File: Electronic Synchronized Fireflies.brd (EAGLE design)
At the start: 100 x 80 mm, 34 parts, among them Q1 NPN/PNP, U2 MSP430G2231/TSSOP-14, X1 22-23-2021, X2 22-23-2031

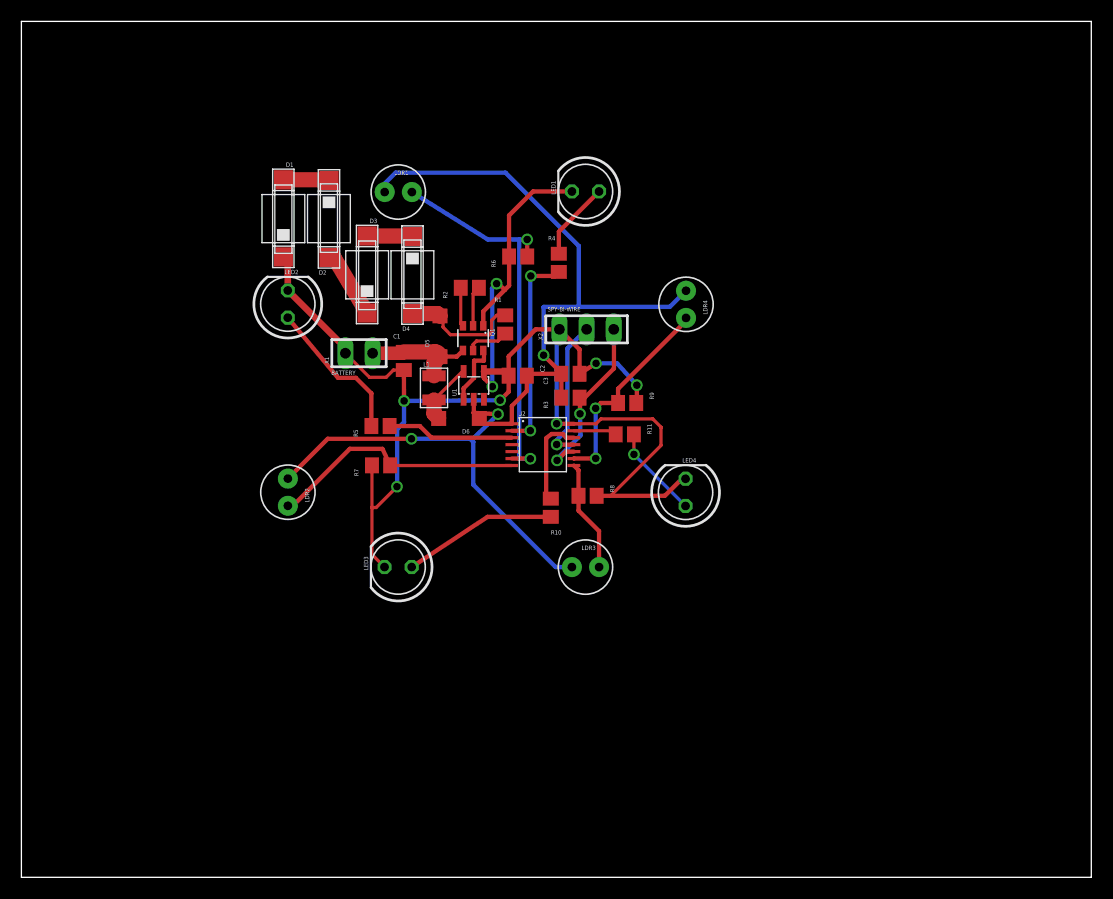
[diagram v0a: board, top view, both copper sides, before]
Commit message: Connections for panel, battery, PCB improvements
v0.3 EECS 399 Spring 2012
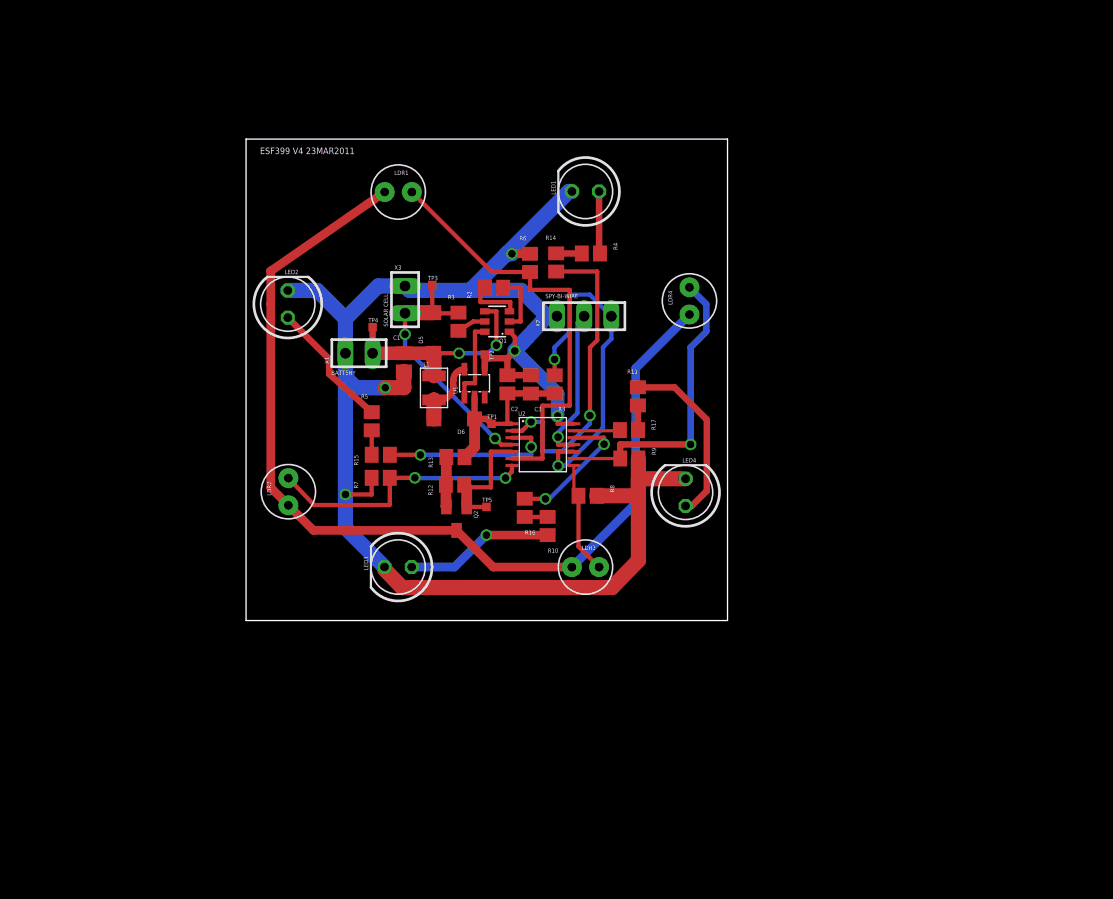
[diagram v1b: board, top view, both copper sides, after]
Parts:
- removed D1, D2, D3, D4: PHOTODIODESMD2, Firefly:PHOTODIODE-SMD2
- added Q2: DMP2035U-7, Firefly:SOT23
- added R12: 20kohm, Firefly:R0805
- added R13, R14, R15, R16, R17: 0ohm, Firefly:R0805
- added TP1, TP2, TP3, TP4, TP5: TPTP08SQ, Firefly:TP08SQ
- added X3: 22-23-2021, Firefly:22-23-2021
- moved R9 5.20 mm to (56.8, 39.1)
- moved R1 4.38 mm to (40.8, 51.9)
- moved C3 3.83 mm to (47.6, 46.1), turned to 90 degrees
- moved R11 3.76 mm to (57.6, 45.0), turned to 270 degrees
- moved R4 3.12 mm to (53.2, 58.3), turned to 180 degrees
- moved Q1 2.73 mm to (44.5, 52.0), turned to 90 degrees
- moved R2 2.27 mm to (44.2, 55.1)
- moved R3 1.93 mm to (49.8, 46.1), turned to 90 degrees
- moved R10 1.73 mm to (49.2, 32.8)
- moved R6 1.26 mm to (47.5, 57.4), turned to 270 degrees
- moved C2 1.26 mm to (45.4, 46.1), turned to 90 degrees
- moved X2 1.25 mm to (52.6, 52.4)
- moved R7 1.17 mm to (33.6, 37.3)
- moved R5 0.93 mm to (32.7, 42.6), turned to 270 degrees
- moved D5 0.66 mm to (38.5, 50.9)
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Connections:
- new net N$25: R11.2, R17.1
- new net N$26: R10.2, R16.1
- net GND: now also TP2.TP, X3.1; no longer D1.P$2
- net N$1: now also LDR1.K, LDR2.K, LDR3.K, LDR4.K, Q2.3; no longer D1.P$1, D2.P$2
- net N$11: now also R14.2; no longer R4.2
- net N$12: now also R15.2; no longer R5.2
- net N$13: now also D5.A, R1.1, TP3.TP, X3.2
- net N$15: now also Q2.2, R12.1, R13.1; no longer U2.5
- net N$19: now also R14.1, R4.2; no longer D3.P$1, D4.P$2
- net N$21: now also R17.2; no longer R11.2
- net N$22: now also R15.1, R5.2; no longer D4.P$1, D5.A, R1.1
- net N$23: now also R16.2; no longer R10.2
- net N$3: now also Q2.1, R12.2, TP5.TP, U2.5; no longer D2.P$1, D3.P$2
- net N$4: now also TP4.TP
- net N$8: now also R13.2, TP1.TP; no longer LDR1.K, LDR2.K, LDR3.K, LDR4.K
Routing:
- net N$8: track 105.9 -> 17.3 mm, vias 3 -> 0
- net N$1: track 4.29 -> 92.6 mm
- net N$13: track 0.00 -> 24.8 mm, vias 0 -> 2
- net N$14: track 16.7 -> 32.1 mm
- net N$11: track 19.0 -> 29.8 mm
- net N$4: track 10.9 -> 21.4 mm, vias 0 -> 2
- net N$22: track 11.4 -> 2.29 mm
- net N$30: track 19.6 -> 28.2 mm, vias 2 -> 1
- net N$32: track 8.69 -> 16.9 mm, vias 1 -> 0
- net N$3: track 6.51 -> 11.6 mm
- net N$12: track 11.9 -> 16.6 mm, vias 0 -> 2
- net N$15: track 0.00 -> 4.69 mm
- net GND: track 145.8 -> 150.3 mm, vias 8 -> 5
- net N$23: track 8.72 -> 13.0 mm, vias 0 -> 2
- net N$17: track 36.9 -> 40.7 mm, vias 2 -> 0
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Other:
- board size 100 x 80 mm -> 45 x 45 mm
- board text added: "ESF399 V4 23MAR2011"
- board text added: "SOLAR CELL"
